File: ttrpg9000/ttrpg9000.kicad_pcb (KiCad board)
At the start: 2 copper layers, 101.6 x 40.6 mm, 35 parts, among them SW1 SW_SPDT, SW2 RotaryEncoder_Switch, SW3 RotaryEncoder_Switch, U1 ATtiny2313A-P, U2 LP2950-3.3_TO92

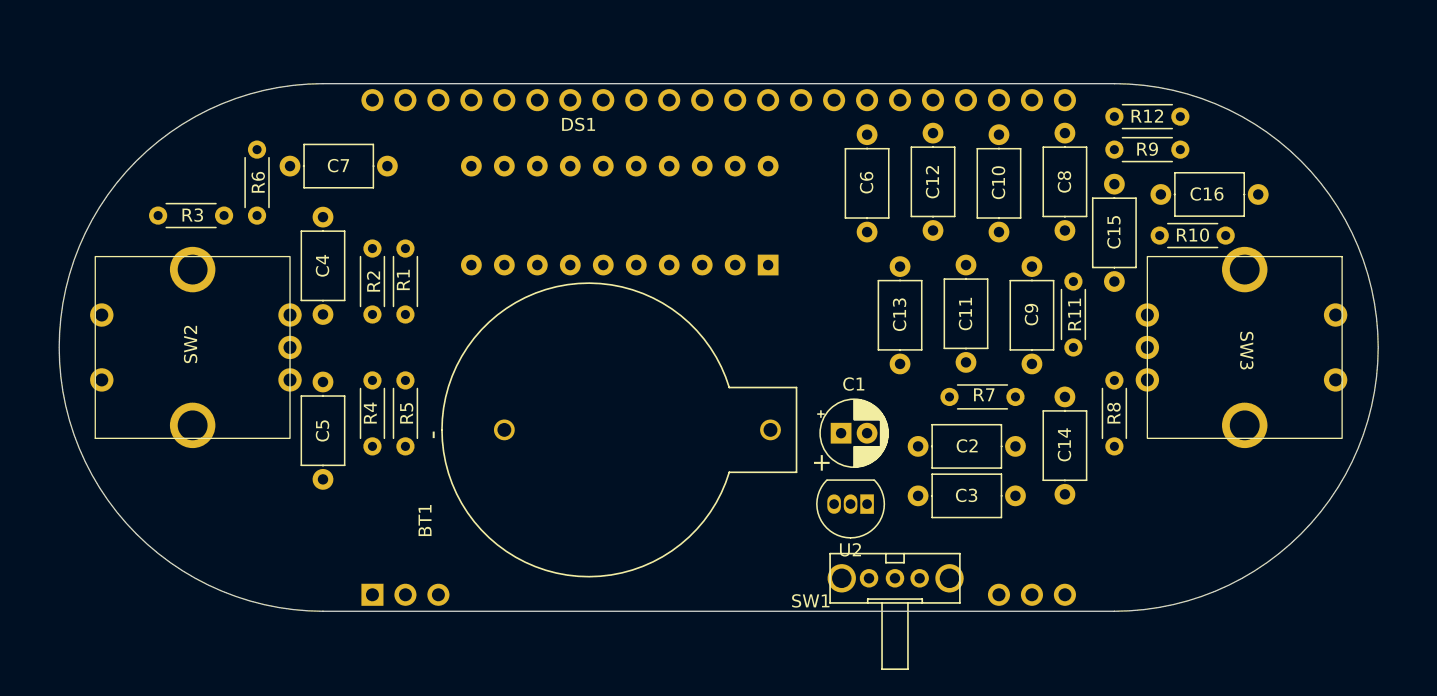
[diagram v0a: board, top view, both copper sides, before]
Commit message: Finalize v0.1 board layout
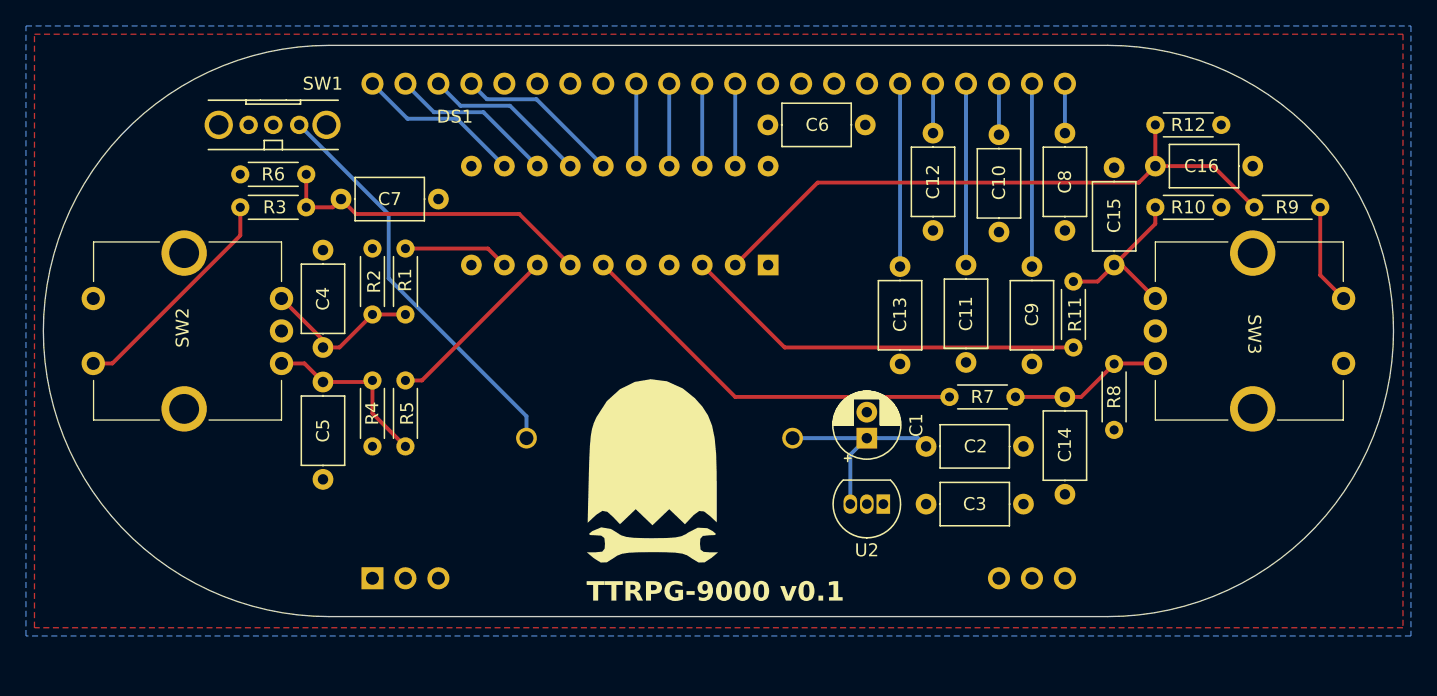
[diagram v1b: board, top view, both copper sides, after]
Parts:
- added G***: LOGO, Project:GhostWrenchLogo, F.Cu at (134.6, 103.5)
- BT1: moved to B.Cu
- moved SW1 59.3 mm to (105.4, 76.8), turned to 180 degrees
- moved DS1 33.5 mm to (139.7, 92.7)
- moved R9 11.7 mm to (186.0, 83.2)
- moved R3 6.36 mm to (102.8, 83.2)
- moved R6 4.94 mm to (107.9, 80.6), turned to 180 degrees
- moved C7 4.68 mm to (110.6, 82.5)
- moved R12 3.22 mm to (173.3, 76.8)
- moved C4 2.54 mm to (109.2, 94.0)
- moved C16 2.23 mm to (173.3, 80.0)
- moved R10 2.20 mm to (178.4, 83.2)
- moved C1 2.02 mm to (151.1, 101.0), turned to 90 degrees
- moved BT1 1.82 mm to (131.4, 101.0), turned to -90 degrees
- moved SW2 1.43 mm to (106.0, 92.7)
- moved SW3 1.41 mm to (173.3, 92.7)
- moved C15 1.27 mm to (170.2, 80.1)
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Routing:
- net Net-(U1-PD0): track 0.00 -> 47.6 mm
- net Net-(BT1--): track 0.00 -> 31.4 mm
- net Net-(U1-PD1): track 0.00 -> 31.2 mm
- net Net-(U1-PD2): track 0.00 -> 30.9 mm
- net Net-(U1-PD3): track 0.00 -> 25.2 mm
- net Net-(R3-Pad1): track 0.00 -> 17.6 mm
- net +6V: track 0.00 -> 16.1 mm
- net Net-(DS1-V4): track 0.00 -> 14.1 mm
- net Net-(DS1-V0): track 0.00 -> 14.1 mm
- net Net-(DS1-V2): track 0.00 -> 14.0 mm
- net Net-(U1-PD4): track 0.00 -> 13.8 mm
- net Net-(C5-Pad2): track 0.00 -> 13.8 mm
- net Net-(C15-Pad2): track 0.00 -> 13.7 mm
- net Net-(DS1-RS): track 0.00 -> 12.8 mm
- net Net-(DS1-R/~{W}): track 0.00 -> 12.8 mm
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- added copper zone on F.Cu, net +3V3
- added copper zone on B.Cu, net GND
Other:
- board size 101.6 x 40.6 mm -> 104 x 44 mm
- board text added: "TTRPG-9000 v0.1"
